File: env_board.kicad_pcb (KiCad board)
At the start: 2 copper layers, 20.7 x 19.2 mm, 22 parts, among them J1 CONN_01X07, J2 BATT_CONN, P1 USB_OTG, Q1 Q_NMOS_GSD, Q2 Q_PMOS_GSD, U1 RFD77101, U2 ENS210, U3 CCS811, U4 AP2204K-3.0, U5 MCP73811T-420I-OT

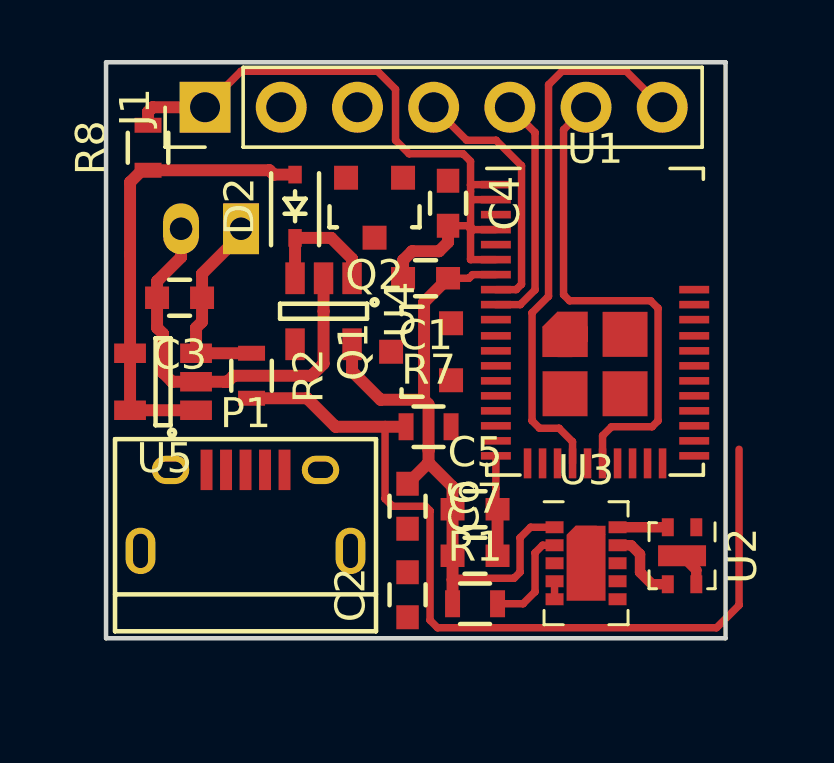
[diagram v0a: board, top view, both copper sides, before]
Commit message: update pcb
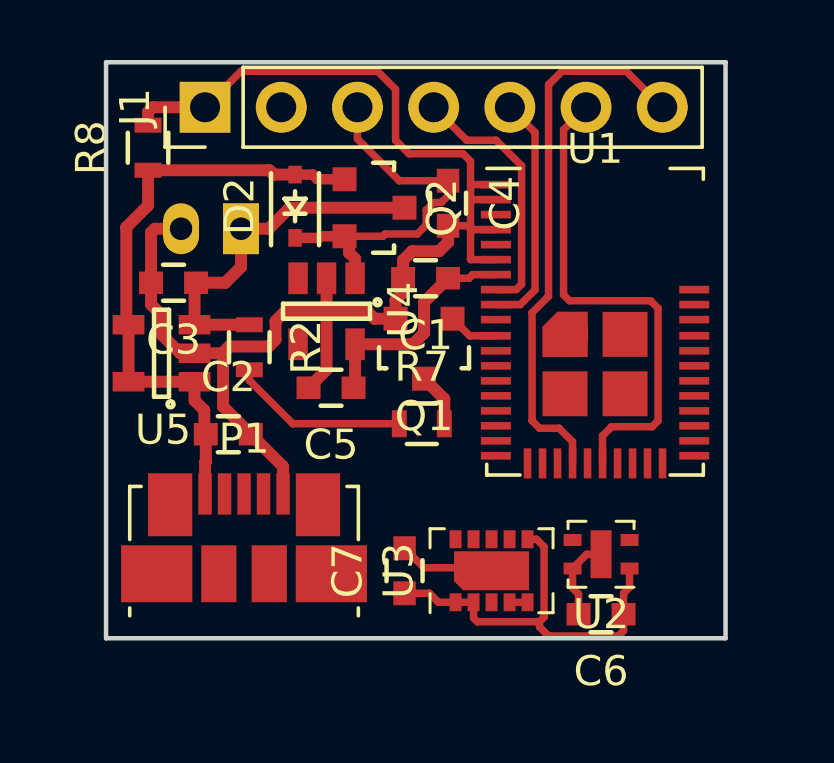
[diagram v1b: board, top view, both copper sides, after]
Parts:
- removed R1: 10k, Resistors_SMD:R_0603
- P1: footprint Connect:USB_Micro-B -> Connectors_USB:USB_Micro-B_Molex_47346-0001
- moved C2 8.02 mm to (152.3, 109.9), turned to 0 degrees
- moved C6 7.39 mm to (164.7, 115.9), turned to 180 degrees
- moved C5 6.28 mm to (155.7, 108.3), turned to 180 degrees
- moved U3 3.16 mm to (161.1, 114.5), turned to 90 degrees
- moved U2 2.70 mm to (164.7, 113.9), turned to 180 degrees
- moved C7 2.40 mm to (158.2, 114.5), turned to 90 degrees
- moved P1 1.90 mm to (152.8, 114.5)
- moved R2 0.95 mm to (153.0, 107.0)
- moved U5 0.95 mm to (150.1, 107.2)
- moved C3 0.54 mm to (150.4, 104.8)
- moved R7 0.25 mm to (158.7, 109.5)
- moved Q1 0.14 mm to (158.8, 107.0), turned to 180 degrees
- moved U4 0.10 mm to (155.6, 105.8)
- turned Q2 to 270 degrees
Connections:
- C4 pad 1: Net-(C4-Pad1) -> VBUS
- D2 pad 1: Net-(C4-Pad1) -> VBUS
- J1 pad 3: VDD -> VBUS
- Q2 pad 2: Net-(C4-Pad1) -> VBUS
- U1 pad 11: (no net) -> /PowerMgmt/BATT_V_EN
- U1 pad 20: /PowerMgmt/BATT_V_EN -> (no net)
- U1 pad 28: (no net) -> /CCS_WAKE
- U3 pad 2: Net-(R1-Pad2) -> VDD
- U3 pad 7: (no net) -> /CCS_WAKE
- U4 pad 1: Net-(C4-Pad1) -> VBUS
- U4 pad 3: Net-(C4-Pad1) -> VBUS
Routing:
- net /PowerMgmt/BATT_V: track 29.2 -> 5.95 mm
- net VBUS: track 0.00 -> 12.7 mm
- net GND: track 42.8 -> 55.3 mm
- net +BATT: track 6.62 -> 12.2 mm
- net Net-(C2-Pad1): track 15.5 -> 20.5 mm
- net Net-(C4-Pad1): track 4.34 -> 0.00 mm
- net Net-(R1-Pad2): track 3.72 -> 0.00 mm
- net /SDA: track 2.56 -> 0.00 mm
- net Net-(Q1-Pad3): track 0.00 -> 1.78 mm
- net /PowerMgmt/BATT_V_EN: track 0.00 -> 1.68 mm
- net /SCL: track 1.68 -> 0.00 mm
- net VDD: track 22.9 -> 21.6 mm
